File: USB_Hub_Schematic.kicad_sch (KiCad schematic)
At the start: 108 parts, among them J1 USB-C, J2 USB-A, U1 USB2517 Chip, U10 TP, U11 TP, U12 TP, U13 TP, U14 TP, U15 TP, U16 TPS25821, U17 TPS25821, U2 3.3V CONV, U3 MUX, U4 USB to microSD, U7 TPS2052B, U9 TP, X3 24MHz Osc

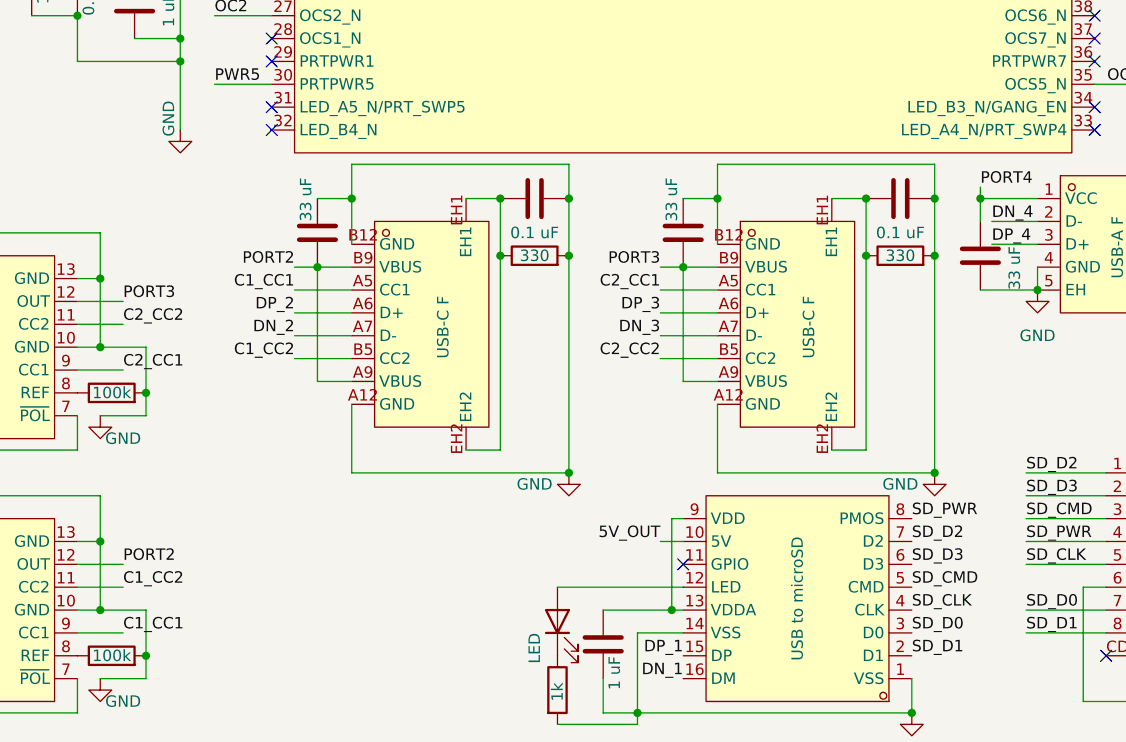
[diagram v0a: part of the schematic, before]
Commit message: Routing draft complete
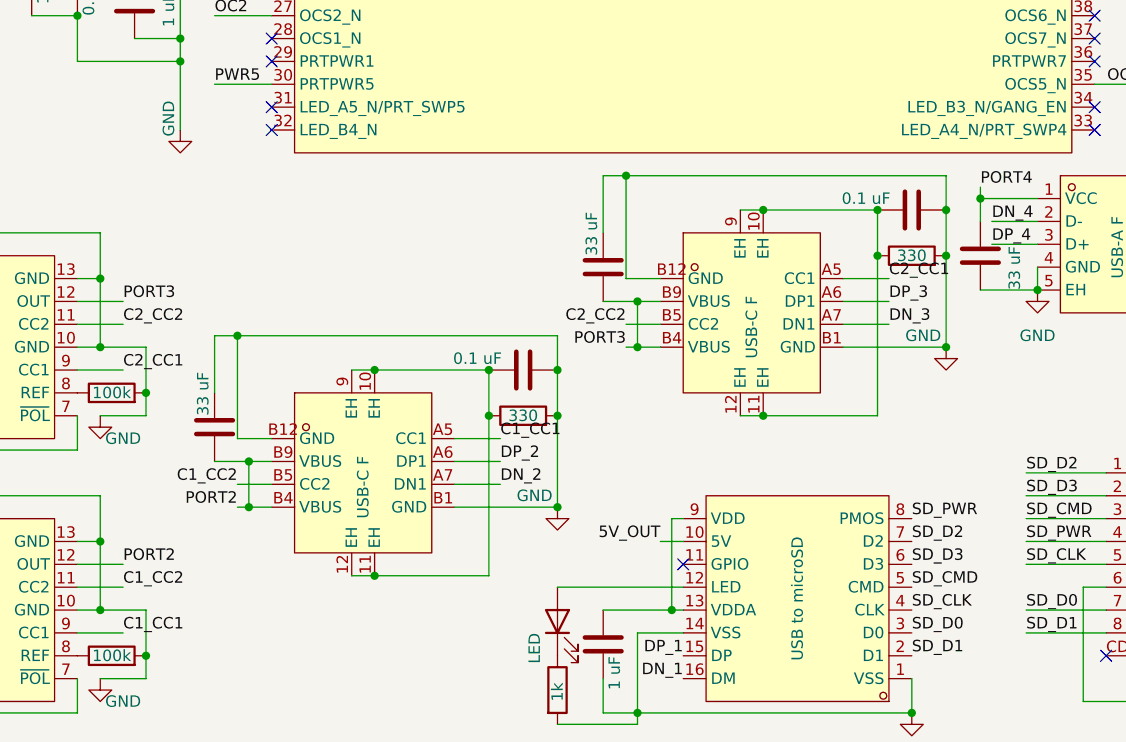
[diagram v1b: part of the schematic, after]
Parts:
- removed C50: 33 uF, Capacitor_SMD:C_0805_2012Metric, symbol Device:C
- removed C51: 0.1 uF, Capacitor_SMD:C_0402_1005Metric, symbol Device:C
- removed R35: 330, Resistor_SMD:R_0603_1608Metric, symbol Device:R
- removed USB1, USB2: USB-C F, lcsc_easyeda:USB-C-SMD_GT-USB-7100A, symbol lcsc_easyeda:GT-USB-7100A
- added C21: 33 uF, Capacitor_SMD:C_0805_2012Metric, symbol Device:C
- added C26: 0.1 uF, Capacitor_SMD:C_0402_1005Metric, symbol Device:C
- added R33: 330, Resistor_SMD:R_0603_1608Metric, symbol Device:R
- added USB3, USB4: USB-C F, lcsc_easyeda:USB-C-SMD_MC-403L68-Z20, symbol lcsc_easyeda:MC-403L68-Z20
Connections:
- net C1_CC1: now also USB3.A5 (CC1)
- net C1_CC2: now also USB3.B5 (CC2)
- net C2_CC1: now also USB4.A5 (CC1)
- net C2_CC2: now also USB4.B5 (CC2)
- net DN_2: now also USB3.A7 (DN1)
- net DN_3: now also USB4.A7 (DN1)
- net DP_2: now also USB3.A6 (DP1)
- net DP_3: now also USB4.A6 (DP1)
- net GND: now also C21.1, C26.2, R33.2, USB3.B1 (GND), USB3.B12 (GND), USB4.B1 (GND), USB4.B12 (GND)
- net PORT2: now also USB3.B4 (VBUS), USB3.B9 (VBUS)
- net PORT3: now also C21.2, USB4.B4 (VBUS), USB4.B9 (VBUS)
- net at C18.1, R32.1: now also USB3.10 (EH), USB3.11 (EH), USB3.12 (EH), USB3.9 (EH)
- new net: C26.1, R33.1, USB4.10 (EH), USB4.11 (EH), USB4.12 (EH), USB4.9 (EH)
